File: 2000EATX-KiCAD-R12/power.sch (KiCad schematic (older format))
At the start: 50 parts, among them CN400 ATX-24, J9003 Case Fan, J9100 POWER_SWITCH, Q9100 MMBT3904, U9000 MC7905, U9101 74HCT14, U9102 74HCT74

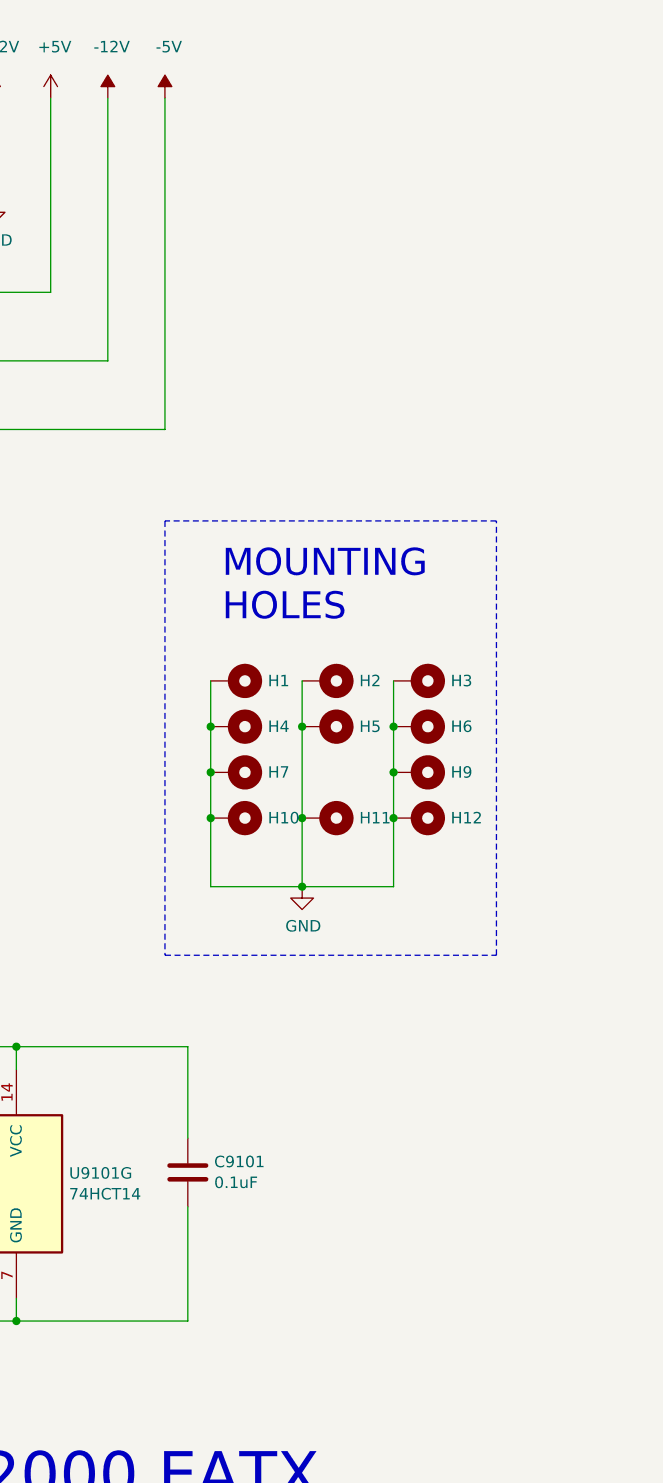
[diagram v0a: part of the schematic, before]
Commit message: Add files via upload
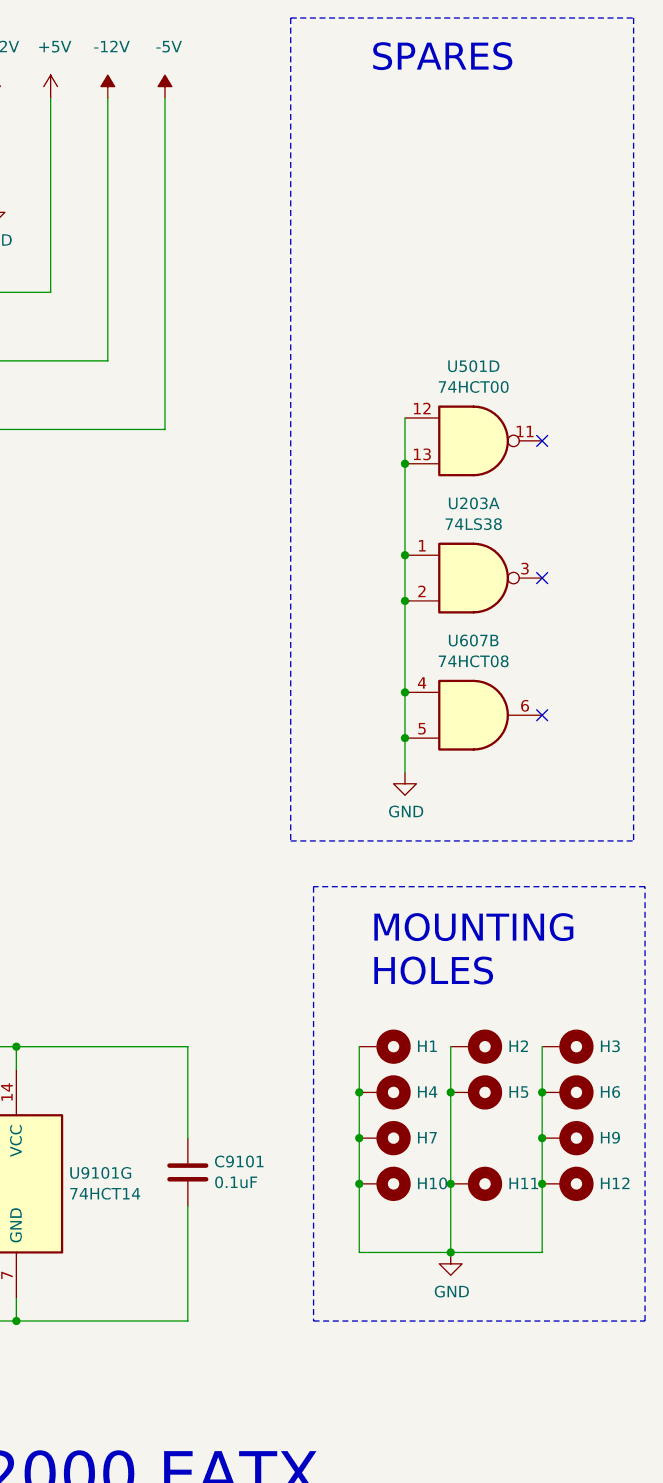
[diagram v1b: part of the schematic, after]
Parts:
- added U203: 74LS38, Package_SO:SOIC-14_3.9x8.7mm_P1.27mm, symbol 74xx:74LS38
- added U501: 74HCT00, Package_SO:SOIC-14_3.9x8.7mm_P1.27mm, symbol 74xx:74LS00
- added U607: 74HCT08, Package_SO:SOIC-14_3.9x8.7mm_P1.27mm, symbol 74xx:74LS08
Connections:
- net GND: now also U203.1, U203.2, U501.12, U501.13, U607.4, U607.5
- no-connect marks 3 -> 6
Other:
- note added: "SPARES"
- moved on the sheet: H1, H10, H11, H12, H2, H3, H4, H5, H6, H7, H9
